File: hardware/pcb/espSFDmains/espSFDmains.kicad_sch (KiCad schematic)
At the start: 22 parts, among them J1 Conn_01x06_Socket, J2 Conn_02x10_Odd_Even, J3 Mains, J4 Mains Motor, U1 WeMos_D1_mini_esp32, U2 TSR_1-2450, U3 SFH617A-1

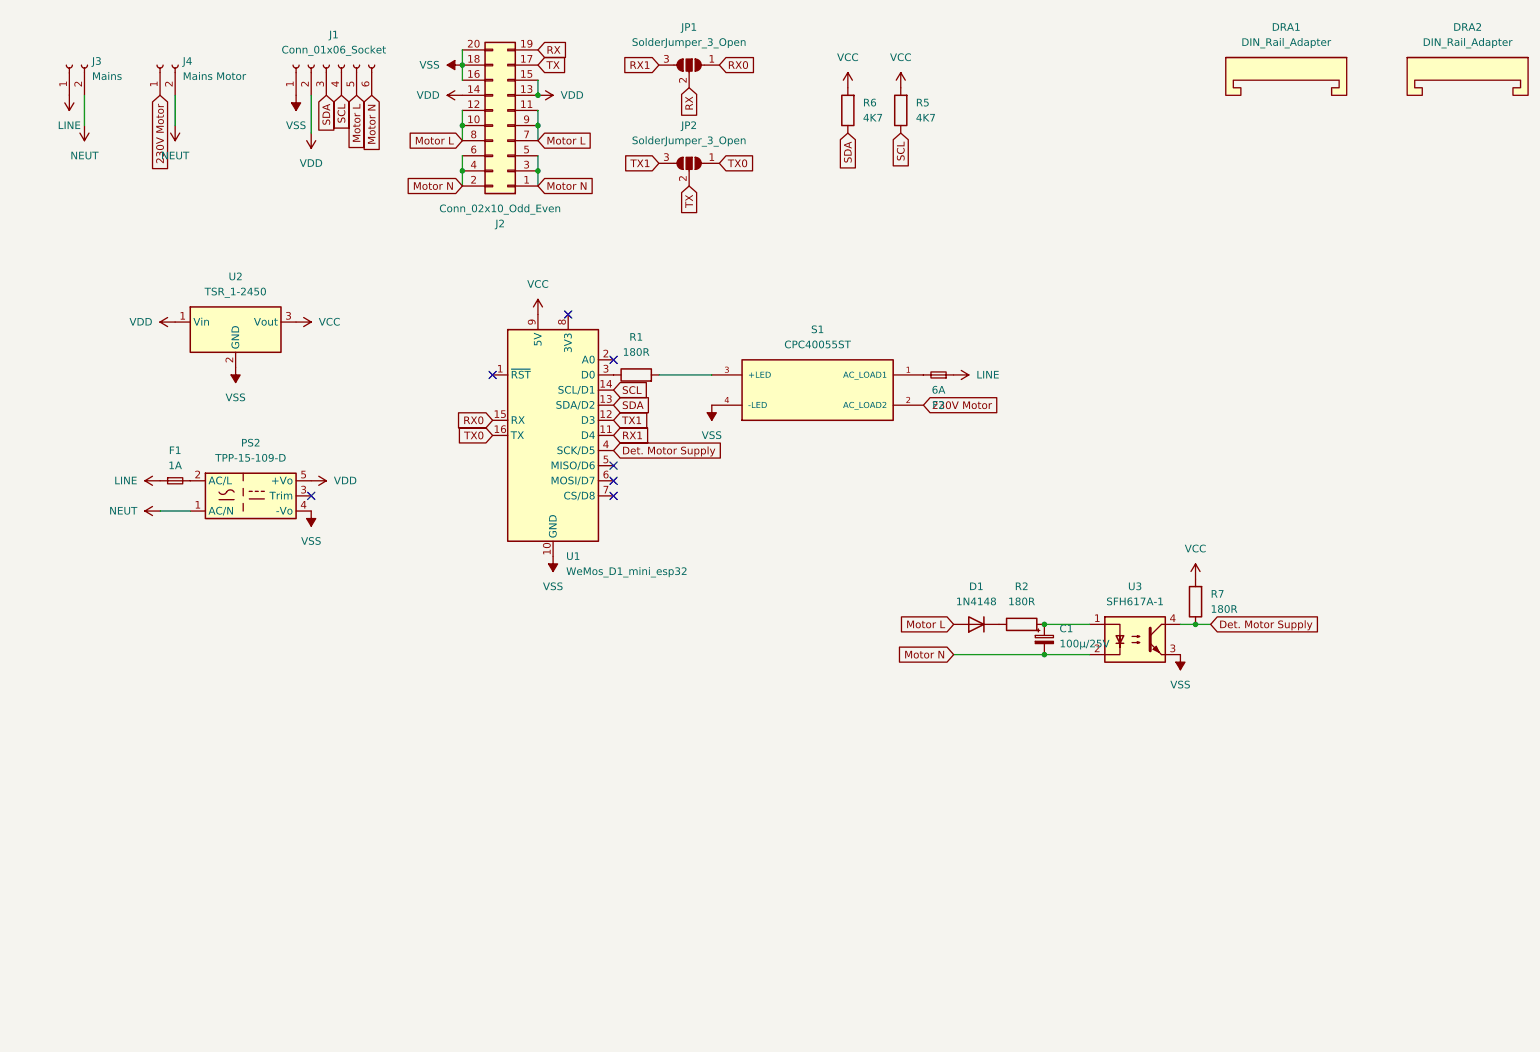
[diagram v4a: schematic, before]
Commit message: bsfnbdfnb
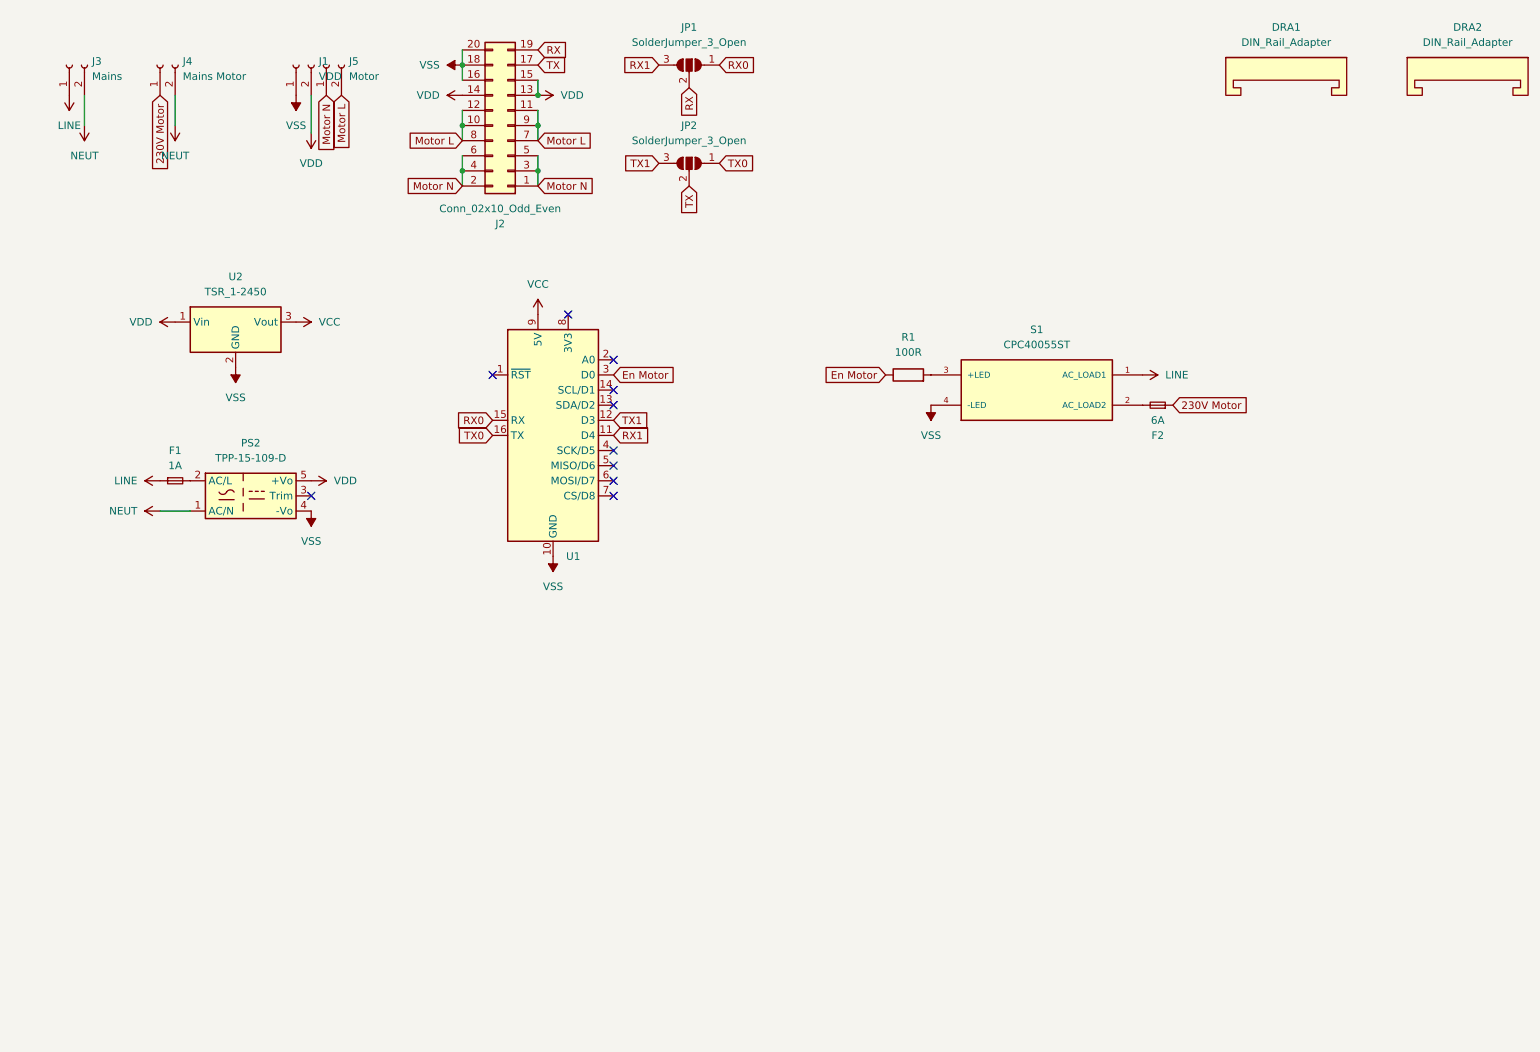
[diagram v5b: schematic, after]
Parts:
- removed C1: 100µ/25V, Capacitor_THT:CP_Radial_D5.0mm_P2.00mm, symbol Device:C_Polarized_Small
- removed D1: 1N4148, Diode_THT:D_DO-35_SOD27_P7.62mm_Horizontal, symbol Diode:1N4148
- removed J1: Conn_01x06_Socket, Connector_Phoenix_MC:PhoenixContact_MC_1,5_6-G-3.81_1x06_P3.81mm_Horizontal, symbol Connector:Conn_01x06_Socket
- removed R2, R7: 180R, Resistor_THT:R_Axial_DIN0204_L3.6mm_D1.6mm_P7.62mm_Horizontal, symbol Device:R
- removed R5, R6: 4K7, Resistor_THT:R_Axial_DIN0204_L3.6mm_D1.6mm_P7.62mm_Horizontal, symbol Device:R
- removed U3: SFH617A-1, Package_DIP:DIP-4_W7.62mm, symbol Isolator:SFH617A-1
- added J1: VDD, Connector_Phoenix_MC:PhoenixContact_MC_1,5_2-G-3.81_1x02_P3.81mm_Horizontal, symbol Connector:Conn_01x02_Socket
- added J5: Motor, Connector_Phoenix_MC:PhoenixContact_MC_1,5_2-G-3.81_1x02_P3.81mm_Horizontal, symbol Connector:Conn_01x02_Socket
- J3, J4: footprint Connector_Phoenix_MSTB:PhoenixContact_MSTBA_2,5_2-G-5,08_1x02_P5.08mm_Horizontal -> Connector_Phoenix_MC:PhoenixContact_MC_1,5_2-G-3.81_1x02_P3.81mm_Horizontal
- R1: value 180R -> 100R
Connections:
- net 230V Motor: now also F2.1; no longer S1.2 (AC_LOAD2)
- net LINE: now also S1.1 (AC_LOAD1); no longer F2.1
- net Motor L: now also J5.2 (Pin_2)
- net Motor N: now also J5.1 (Pin_1)
- net VDD: now also J1.2 (Pin_2)
- net VSS: now also J1.1 (Pin_1)
- net En Motor: now reaches R1.1, U1.3 (D0)
- net at F2.2: now also S1.2 (AC_LOAD2); no longer S1.1 (AC_LOAD1)
- net Det. Motor Supply: no longer names the net of U1.4 (SCK/D5)
- net SCL: no longer names the net of U1.14 (SCL/D1)
- net SDA: no longer names the net of U1.13 (SDA/D2)
- no-connect marks 7 -> 10
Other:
- moved on the sheet: F2, R1, S1

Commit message: PCB V1.2
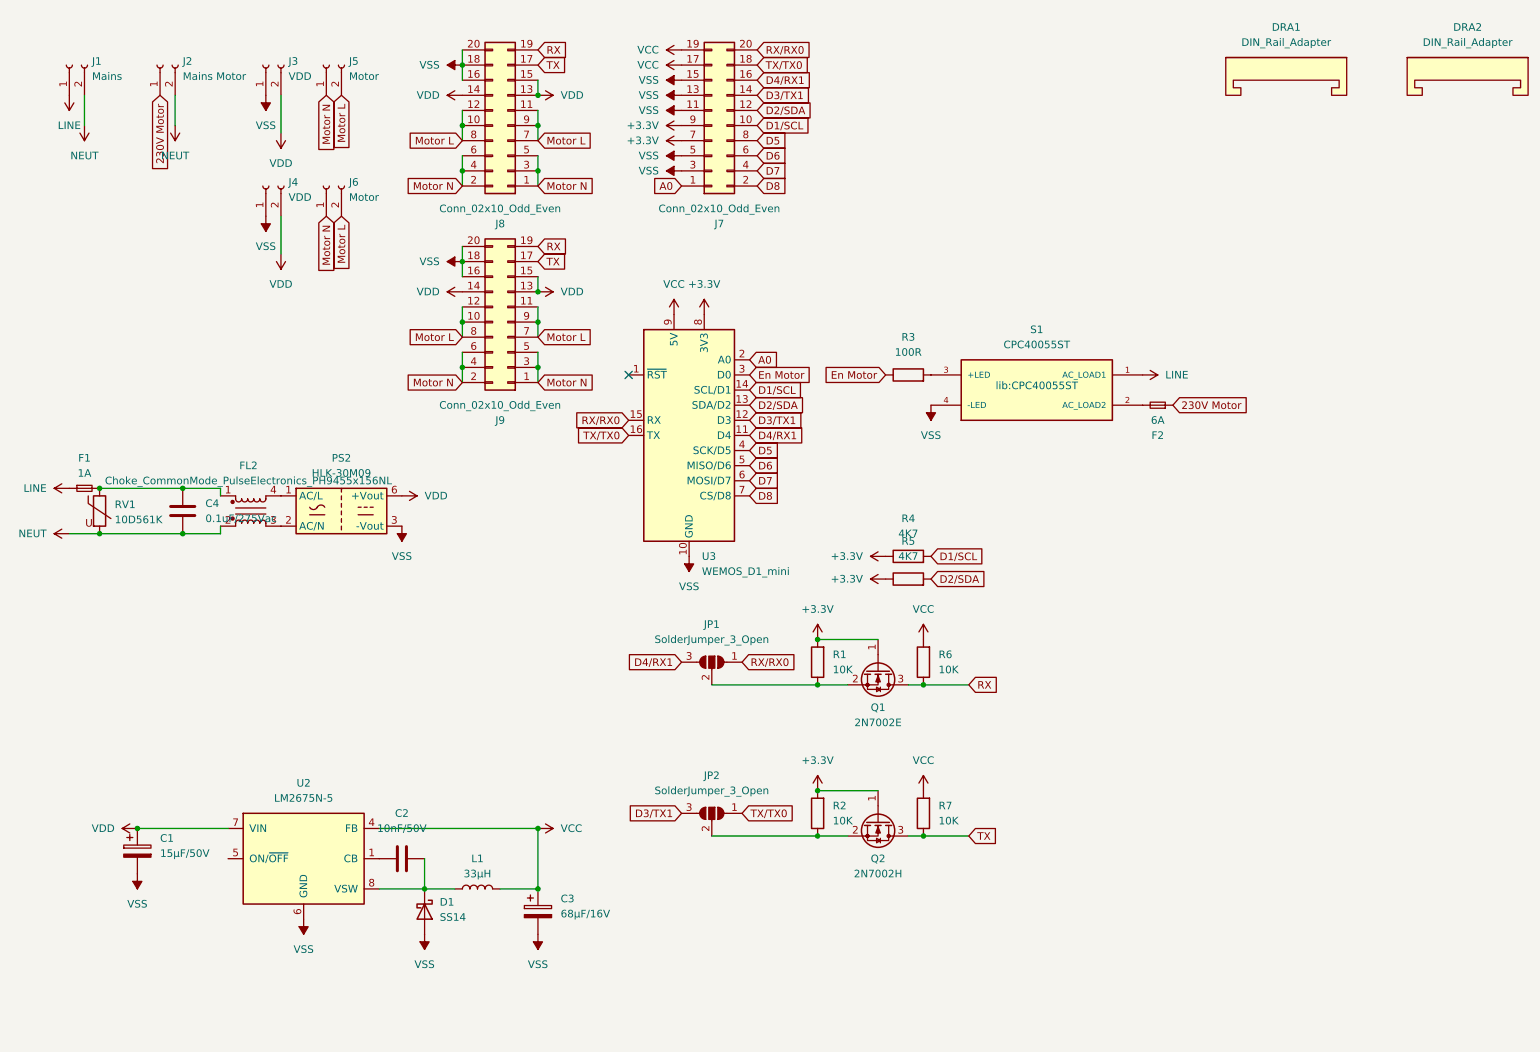
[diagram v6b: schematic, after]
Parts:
- removed PS2: TPP-15-109-D, Converter_ACDC:Converter_ACDC_TRACO_TPP-15-1xx-D_THT, symbol Converter_ACDC:TPP-15-109-D
- removed U1: WeMos_D1_mini_esp32, Module:WEMOS_D1_mini_light, symbol MCU_Module:WeMos_D1_mini
- removed U2: TSR_1-2450, Converter_DCDC:Converter_DCDC_TRACO_TSR-1_THT, symbol Regulator_Switching:TSR_1-2450
- added C1: 15µF/50V, Capacitor_Tantalum_SMD:CP_EIA-7343-43_Kemet-X, symbol Device:C_Polarized
- added C2: 10nF/50V, Capacitor_SMD:C_0805_2012Metric, symbol Device:C
- added C3: 68µF/16V, Capacitor_Tantalum_SMD:CP_EIA-7343-43_Kemet-X, symbol Device:C_Polarized
- added C4: 0.1uF/275Vac, Capacitor_THT:C_Rect_L16.5mm_W5.0mm_P15.00mm_MKT, symbol Device:C
- added D1: SS14, Diode_SMD:D_SMA, symbol Diode:SS14
- added FL2: Choke_CommonMode_PulseElectronics_PH9455x156NL, Inductor_THT:L_CommonMode_PulseElectronics_PH9455xxx6NL_2, symbol Filter:Choke_CommonMode_PulseElectronics_PH9455x156NL
- added J4: VDD, Connector_Phoenix_MC:PhoenixContact_MCV_1,5_2-G-3.81_1x02_P3.81mm_Vertical, symbol Connector:Conn_01x02_Socket
- added J6: Motor, Connector_Phoenix_MC:PhoenixContact_MCV_1,5_2-G-3.81_1x02_P3.81mm_Vertical, symbol Connector:Conn_01x02_Socket
- added J7, J9: Conn_02x10_Odd_Even, Connector_IDC:IDC-Header_2x10_P2.54mm_Vertical, symbol Connector_Generic:Conn_02x10_Odd_Even
- added L1: 33µH, Inductor_SMD:L_Chilisin_BMRB00060650, symbol Device:L
- added PS2: HLK-30M09, Converter_ACDC:Converter_ACDC_Hi-Link_HLK-30Mxx, symbol Converter_ACDC:HLK-30M09
- added Q1: 2N7002E, Package_TO_SOT_SMD:SOT-23, symbol Transistor_FET:2N7002E
- added Q2: 2N7002H, Package_TO_SOT_SMD:SOT-23, symbol Transistor_FET:2N7002H
- added R1, R2, R6, R7: 10K, Resistor_SMD:R_0603_1608Metric, symbol Device:R
- added R4, R5: 4K7, Resistor_THT:R_Axial_DIN0204_L3.6mm_D1.6mm_P7.62mm_Horizontal, symbol Device:R
- added RV1: 10D561K, Varistor:RV_Disc_D9mm_W6.1mm_P5mm, symbol Device:Varistor
- added U2: LM2675N-5, Package_SO:SOIC-8_3.9x4.9mm_P1.27mm, symbol Regulator_Switching:LM2675N-5
- added U3: WEMOS_D1_mini, RF_Module:WEMOS_D1_mini_light, symbol RF_Module:WEMOS_D1_mini
- DRA1, DRA2: footprint Library:DINRailAdapter_3xM3_PhoenixContact_1201578 -> MountingEquipment:DINRailAdapter_3xM3_PhoenixContact_1201578
- J1: renamed from J3; footprint Connector_Phoenix_MC:PhoenixContact_MC_1,5_2-G-3.81_1x02_P3.81mm_Horizontal -> Connector_Phoenix_MC:PhoenixContact_MCV_1,5_2-G-3.81_1x02_P3.81mm_Vertical
- J2: renamed from J4; footprint Connector_Phoenix_MC:PhoenixContact_MC_1,5_2-G-3.81_1x02_P3.81mm_Horizontal -> Connector_Phoenix_MC:PhoenixContact_MCV_1,5_2-G-3.81_1x02_P3.81mm_Vertical
- J3: renamed from J1; footprint Connector_Phoenix_MC:PhoenixContact_MC_1,5_2-G-3.81_1x02_P3.81mm_Horizontal -> Connector_Phoenix_MC:PhoenixContact_MCV_1,5_2-G-3.81_1x02_P3.81mm_Vertical
- J5: footprint Connector_Phoenix_MC:PhoenixContact_MC_1,5_2-G-3.81_1x02_P3.81mm_Horizontal -> Connector_Phoenix_MC:PhoenixContact_MCV_1,5_2-G-3.81_1x02_P3.81mm_Vertical
- JP1, JP2: footprint Library:SolderJumper-3_P1.3mm_Open_Pad1.0x1.5mm no silk -> Connector_PinHeader_2.54mm:PinHeader_1x03_P2.54mm_Vertical
- renumbered J2 to J8, R1 to R3
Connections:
- net En Motor: now also U3.3 (D0)
- net Motor L: now also J6.2 (Pin_2), J9.10 (Pin_10), J9.11 (Pin_11), J9.12 (Pin_12), J9.7 (Pin_7), J9.8 (Pin_8), J9.9 (Pin_9)
- net Motor N: now also J6.1 (Pin_1), J9.1 (Pin_1), J9.2 (Pin_2), J9.3 (Pin_3), J9.4 (Pin_4), J9.5 (Pin_5), J9.6 (Pin_6)
- net NEUT: now also C4.2, FL2.2, RV1.2
- net RX: now also J9.19 (Pin_19), Q1.3 (D), R6.1; no longer JP1.2 (C)
- net TX: now also J9.17 (Pin_17), Q2.3 (D), R7.1; no longer JP2.2 (C)
- net VCC: now also C3.1, J7.17 (Pin_17), J7.19 (Pin_19), L1.2, R6.2, R7.2, U2.4 (FB), U3.9 (5V)
- net VDD: now also C1.1, J4.2 (Pin_2), J9.13 (Pin_13), J9.14 (Pin_14), J9.15 (Pin_15), PS2.6 (+Vout), U2.7 (VIN)
- net VSS: now also C1.2, C3.2, D1.2 (A), J4.1 (Pin_1), J7.11 (Pin_11), J7.13 (Pin_13), J7.15 (Pin_15), J7.3 (Pin_3), J7.5 (Pin_5), J9.16 (Pin_16), J9.18 (Pin_18), J9.20 (Pin_20), PS2.3 (-Vout), U2.6 (GND), U3.10 (GND)
- net at F1.2: now also C4.1, FL2.1, RV1.1
- net RX0 renamed RX/RX0
- net RX/RX0: now also J7.20 (Pin_20), U3.15 (RX)
- net RX1 renamed D4/RX1
- net D4/RX1: now also J7.16 (Pin_16), U3.11 (D4)
- net TX0 renamed TX/TX0
- net TX/TX0: now also J7.18 (Pin_18), U3.16 (TX)
- net TX1 renamed D3/TX1
- net D3/TX1: now also J7.14 (Pin_14), U3.12 (D3)
- new net: JP2.2 (C), Q2.2 (S), R2.1
- new net: C2.2, D1.1 (K), L1.1, U2.8 (VSW)
- new net: C2.1, U2.1 (CB)
- new net: FL2.4, PS2.1 (AC/L)
- new net: FL2.3, PS2.2 (AC/N)
- new net: JP1.2 (C), Q1.2 (S), R1.1
- new net +3.3V: J7.7 (Pin_7), J7.9 (Pin_9), Q1.1 (G), Q2.1 (G), R1.2, R2.2, R4.1, R5.1, U3.8 (3V3)
- new net A0: J7.1 (Pin_1), U3.2 (A0)
- new net D1/SCL: J7.10 (Pin_10), R4.2, U3.14 (SCL/D1)
- new net D2/SDA: J7.12 (Pin_12), R5.2, U3.13 (SDA/D2)
- new net D5: J7.8 (Pin_8), U3.4 (SCK/D5)
- new net D6: J7.6 (Pin_6), U3.5 (MISO/D6)
- new net D7: J7.4 (Pin_4), U3.6 (MOSI/D7)
- new net D8: J7.2 (Pin_2), U3.7 (CS/D8)
- no-connect marks 10 -> 1
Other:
- moved on the sheet: F1, J3, JP1, JP2

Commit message: jfgj
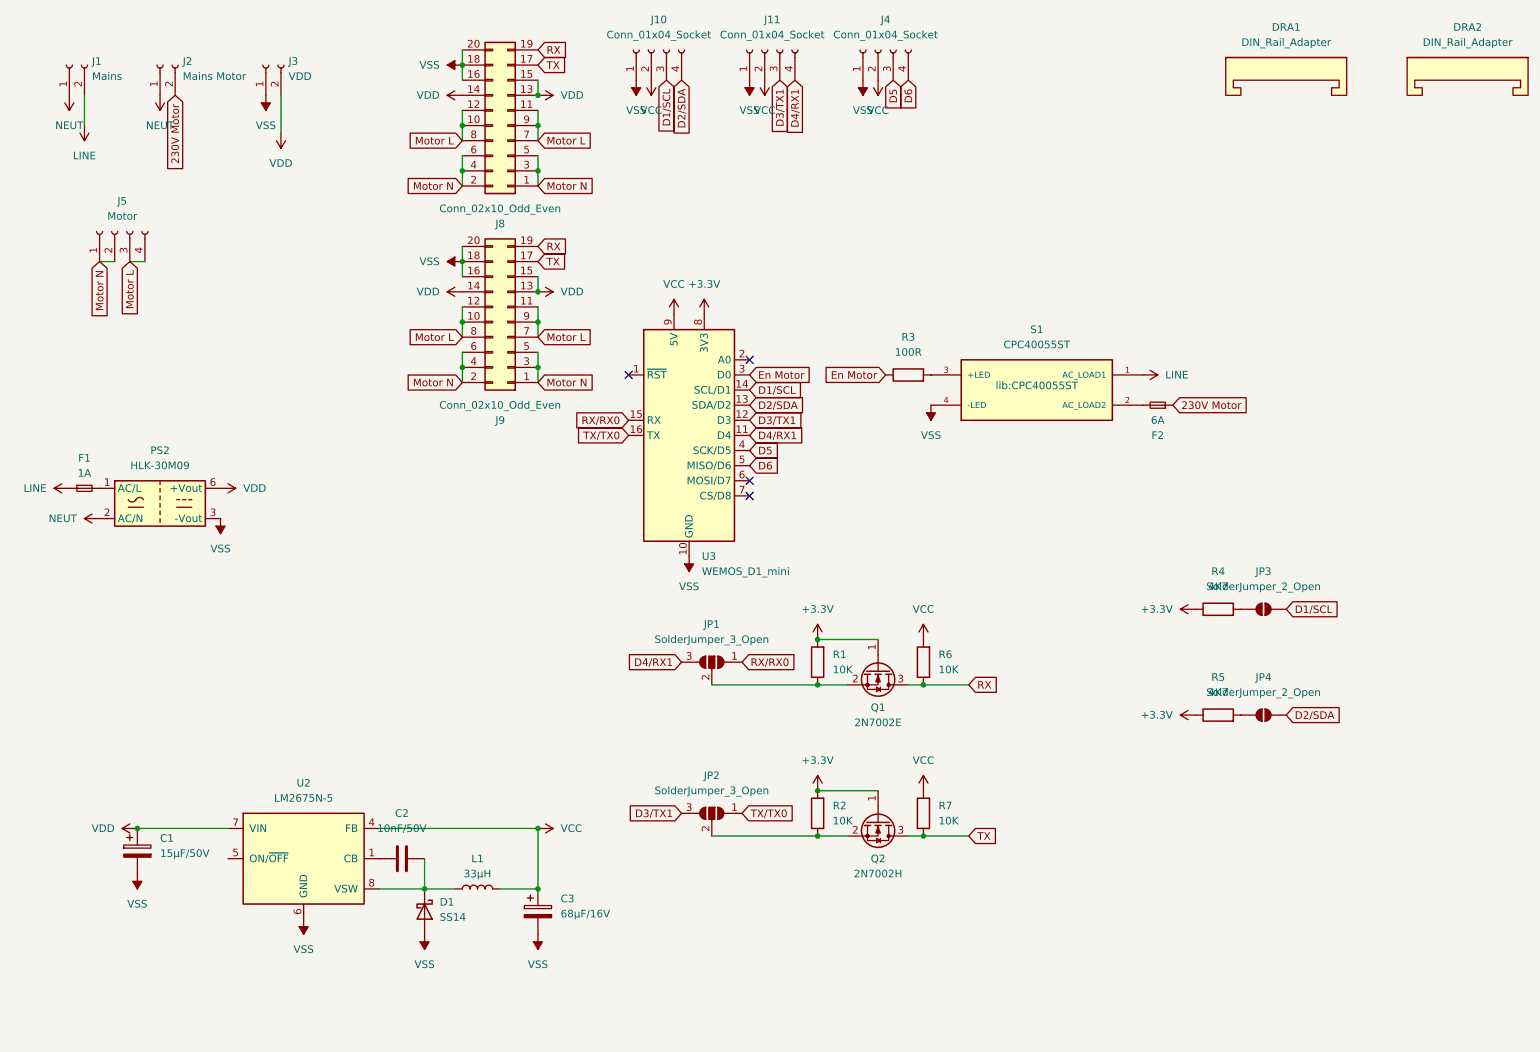
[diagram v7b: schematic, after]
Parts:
- removed C4: 0.1uF/275Vac, Capacitor_THT:C_Rect_L16.5mm_W5.0mm_P15.00mm_MKT, symbol Device:C
- removed FL2: Choke_CommonMode_PulseElectronics_PH9455x156NL, Inductor_THT:L_CommonMode_PulseElectronics_PH9455xxx6NL_2, symbol Filter:Choke_CommonMode_PulseElectronics_PH9455x156NL
- removed J4: VDD, Connector_Phoenix_MC:PhoenixContact_MCV_1,5_2-G-3.81_1x02_P3.81mm_Vertical, symbol Connector:Conn_01x02_Socket
- removed J5, J6: Motor, Connector_Phoenix_MC:PhoenixContact_MCV_1,5_2-G-3.81_1x02_P3.81mm_Vertical, symbol Connector:Conn_01x02_Socket
- removed J7: Conn_02x10_Odd_Even, Connector_IDC:IDC-Header_2x10_P2.54mm_Vertical, symbol Connector_Generic:Conn_02x10_Odd_Even
- removed RV1: 10D561K, Varistor:RV_Disc_D9mm_W6.1mm_P5mm, symbol Device:Varistor
- added J10, J11, J4: Conn_01x04_Socket, Connector_Phoenix_MC:PhoenixContact_MCV_1,5_4-G-3.81_1x04_P3.81mm_Vertical, symbol Connector:Conn_01x04_Socket
- added J5: Motor, Connector_Phoenix_MC:PhoenixContact_MCV_1,5_4-G-3.81_1x04_P3.81mm_Vertical, symbol Connector:Conn_01x04_Socket
- added JP3, JP4: SolderJumper_2_Open, Jumper:SolderJumper-2_P1.3mm_Open_Pad1.0x1.5mm, symbol Jumper:SolderJumper_2_Open
- JP1, JP2: footprint Connector_PinHeader_2.54mm:PinHeader_1x03_P2.54mm_Vertical -> Jumper:SolderJumper-3_P1.3mm_Open_Pad1.0x1.5mm
- R3, R4, R5: footprint Resistor_THT:R_Axial_DIN0204_L3.6mm_D1.6mm_P7.62mm_Horizontal -> Resistor_SMD:R_0603_1608Metric
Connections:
- net 230V Motor: now also J2.2 (Pin_2); no longer J2.1 (Pin_1)
- net D1/SCL: now also J10.3 (Pin_3), JP3.2 (B); no longer R4.2
- net D2/SDA: now also J10.4 (Pin_4), JP4.2 (B); no longer R5.2
- net D3/TX1: now also J11.3 (Pin_3)
- net D4/RX1: now also J11.4 (Pin_4)
- net D5: now also J4.3 (Pin_3)
- net D6: now also J4.4 (Pin_4)
- net LINE: now also J1.2 (Pin_2); no longer J1.1 (Pin_1)
- net Motor L: now also J5.3 (Pin_3), J5.4 (Pin_4)
- net Motor N: now also J5.1 (Pin_1), J5.2 (Pin_2)
- net NEUT: now also J1.1 (Pin_1), J2.1 (Pin_1), PS2.2 (AC/N); no longer J1.2 (Pin_2), J2.2 (Pin_2)
- net VCC: now also J10.2 (Pin_2), J11.2 (Pin_2), J4.2 (Pin_2)
- net VSS: now also J10.1 (Pin_1), J11.1 (Pin_1), J4.1 (Pin_1)
- net at PS2.1 (AC/L): now also F1.2
- net A0: no longer names the net of U3.2 (A0)
- net D7: no longer names the net of U3.6 (MOSI/D7)
- net D8: no longer names the net of U3.7 (CS/D8)
- new net: JP3.1 (A), R4.2
- new net: JP4.1 (A), R5.2
- no-connect marks 1 -> 4
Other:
- moved on the sheet: PS2, R4, R5
